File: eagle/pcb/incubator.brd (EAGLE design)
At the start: 99.1 x 63.5 mm, 57 parts, among them IC1 MCP1703-50, J2 RJ12RIGHTANGLE-I2C, J7 22--02, Q1 BSP75, Q5 BSP75, X2 8MHz, X4 MINI-USB

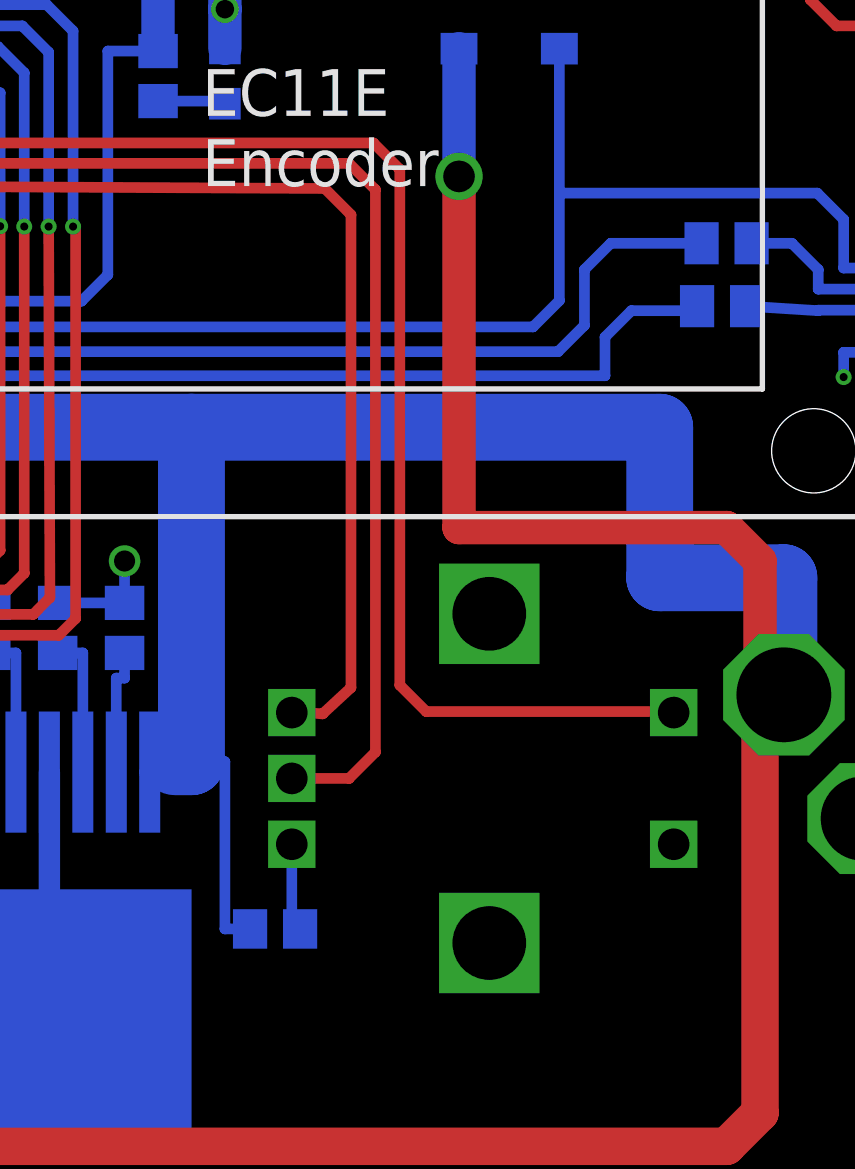
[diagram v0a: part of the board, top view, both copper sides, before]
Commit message: version 1.1
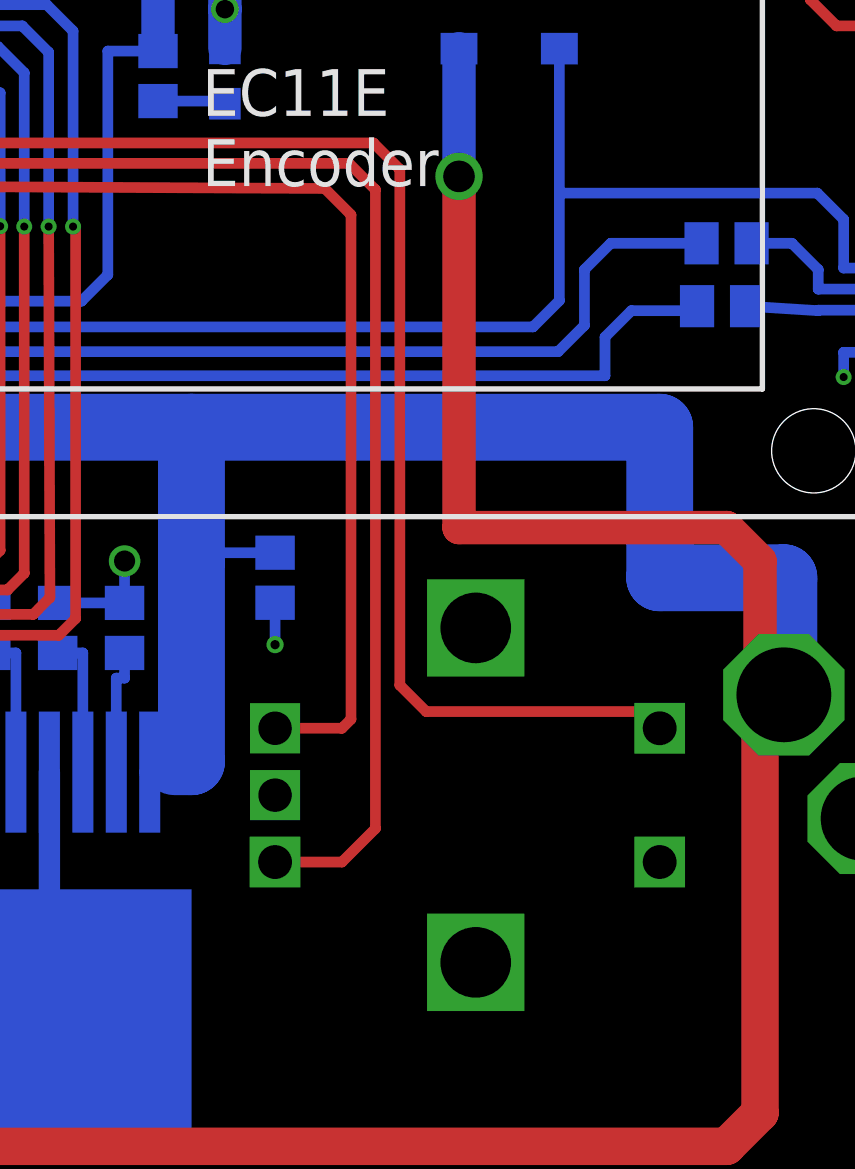
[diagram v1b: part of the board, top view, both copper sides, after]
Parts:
- U$1: value EC11E -> ROTARYENCODER; device lpatiny:EC11E -> RotaryEncoder:ROTARYENCODER
- moved CX4 13.3 mm to (66.7, 22.9), turned to 90 degrees
- moved U$1 7.65 mm to (74.9, 14.6), turned to 0 degrees
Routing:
- net +12V: track 255.9 -> 250.8 mm
- net RX: track 68.9 -> 72.6 mm
- net GND: track 116.7 -> 114.7 mm, vias 17 -> 18
- net TX: track 65.0 -> 66.6 mm
